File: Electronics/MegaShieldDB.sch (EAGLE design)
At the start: 44 parts, among them IC2 MCP4802, IC3 MCP4802, IC4 4013N, Q1 BF199, Q5 BF199, X1 M25-HD-20, X2 Cruise Computers, X4 Steer, X5 Brake

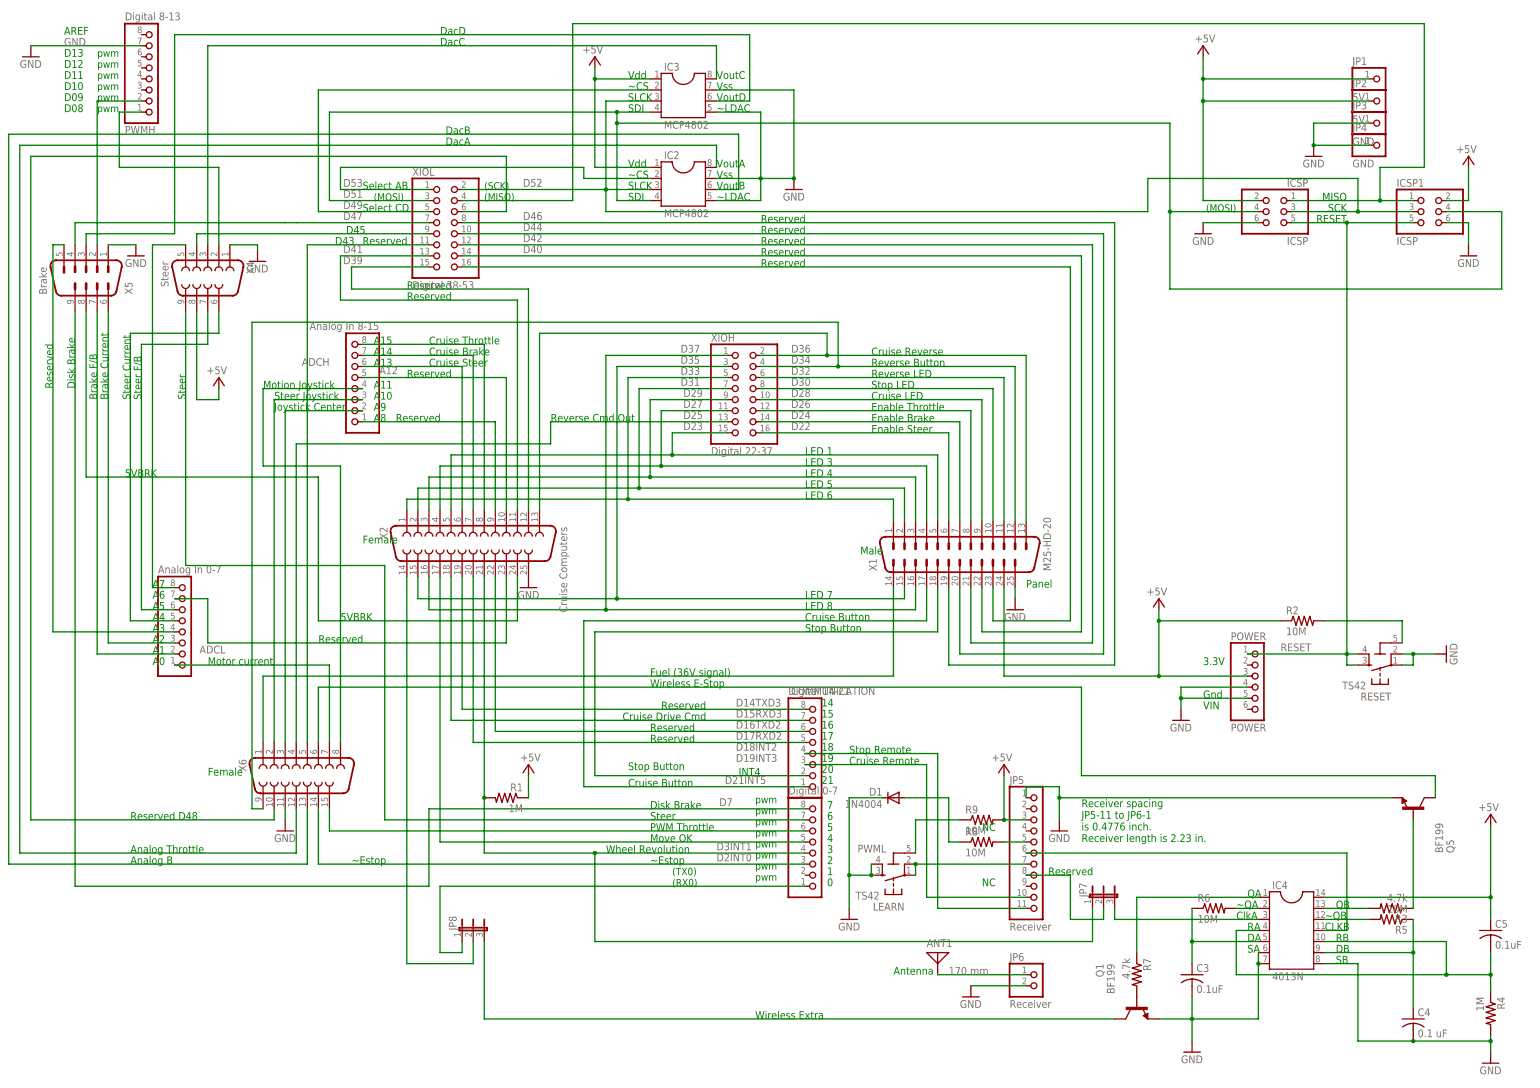
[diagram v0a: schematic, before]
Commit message: update to Sourceforge 123
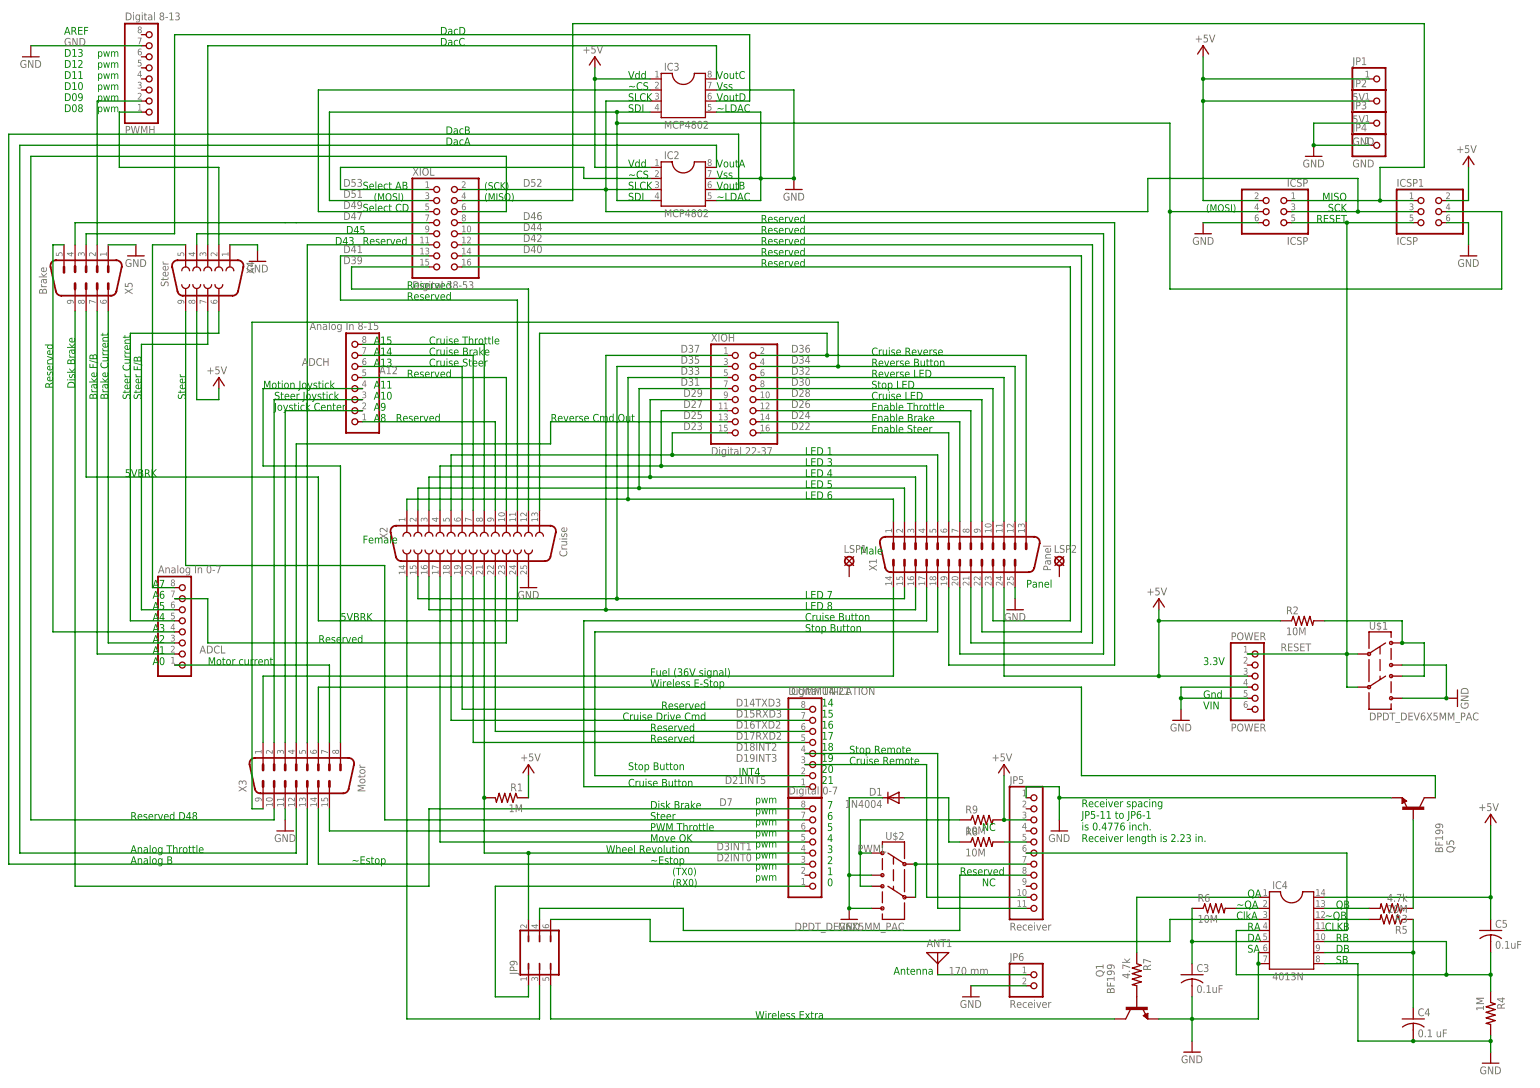
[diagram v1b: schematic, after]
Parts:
- removed JP7, JP8: (no value), jumper:JP2E
- removed LEARN, RESET: TS42, st-mod v1.4:TS42
- removed X6: (no value), con-subd:F15H
- added JP9: (no value), jumper:JP3Q
- added LSP1, LSP2: LSP13, solpad:LSP13
- added U$1, U$2: DPDT_DEV6X5MM_PAC, elcanoParts:DPDT_DEV6X5MM_PAC
- added X3: Motor, con-subd:M15-182
- X1: value M25-HD-20 -> Panel
- X2: value Cruise Computers -> Cruise
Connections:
- net A0: now also X3.7; no longer X6.7
- net A10: now also X3.2; no longer X6.2
- net A11: now also X3.8; no longer X6.8
- net A9: now also X3.3; no longer X6.3
- net CLKA: now also JP9.6; no longer JP7.3
- net D0RX0: now also JP9.1; no longer JP8.1
- net D25: now also X3.4; no longer X6.4
- net D2INT0: now also X3.14; no longer X6.14
- net D34: now also X3.9; no longer X6.9
- net D3INT1: now also JP9.2; no longer JP7.1
- net D43: now also X3.5; no longer X6.5
- net D48: now also X3.10; no longer X6.10
- net D5: now also X3.15; no longer X6.15
- net DACA: now also X3.12; no longer X6.12
- net DACB: now also X3.13; no longer X6.13
- net FUEL: now also X3.1; no longer X6.1
- net GND: now also U$1.3, U$1.6, U$2.3, U$2.6, X3.11; no longer LEARN.3, LEARN.4, RESET.1, RESET.2, X6.11
- net N$10: now also U$2.1, U$2.4; no longer LEARN.5-GND
- net N$28: now also U$2.2, U$2.5; no longer LEARN.1, LEARN.2
- net N$6: now also U$1.1, U$1.4; no longer RESET.5-GND
- net RESET: now also U$1.2, U$1.5; no longer RESET.3, RESET.4
- net WL2: now also JP9.4; no longer JP7.2
- net WLES: now also X3.6; no longer X6.6
- net WLXCOLL: now also JP9.5; no longer JP8.3
- net X2-14: now also JP9.3; no longer JP8.2
